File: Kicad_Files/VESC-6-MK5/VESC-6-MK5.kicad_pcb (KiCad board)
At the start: 4 copper layers, 105.9 x 102.5 mm, 151 parts, among them P1 USB_OTG, P10 PH_C, P11 SUPPLY, P12 GND, P2 CAN, P4 HALL_ENC, P5 COMM, P6 SERVO, P7 SWD, P8 PH_A, P9 PH_B, Q1 IRF7749, Q2 IRF7749, Q3 IRF7749, Q4 IRF7749, Q5 IRF7749, Q6 IRF7749, Q7 DMN62D0UW-7, U1 STM32F405RGTx, U10 MC74VHC1GT66, U11 SENS_VOLT, U12 MC74VHC1GT66, U13 MC74VHC1GT66, U14 MC74VHC1GT66DF1G, U15 MC74VHC1GT66DF1G, U16 MC74VHC1GT66DF1G, U3 DRV8301DCA, U4 TJA1051TK-3, U5 AD8418, U6 AD8418, U7 AD8418, U8 TC2117-3.3VEBTR, U9 BMI160, Y1 8M

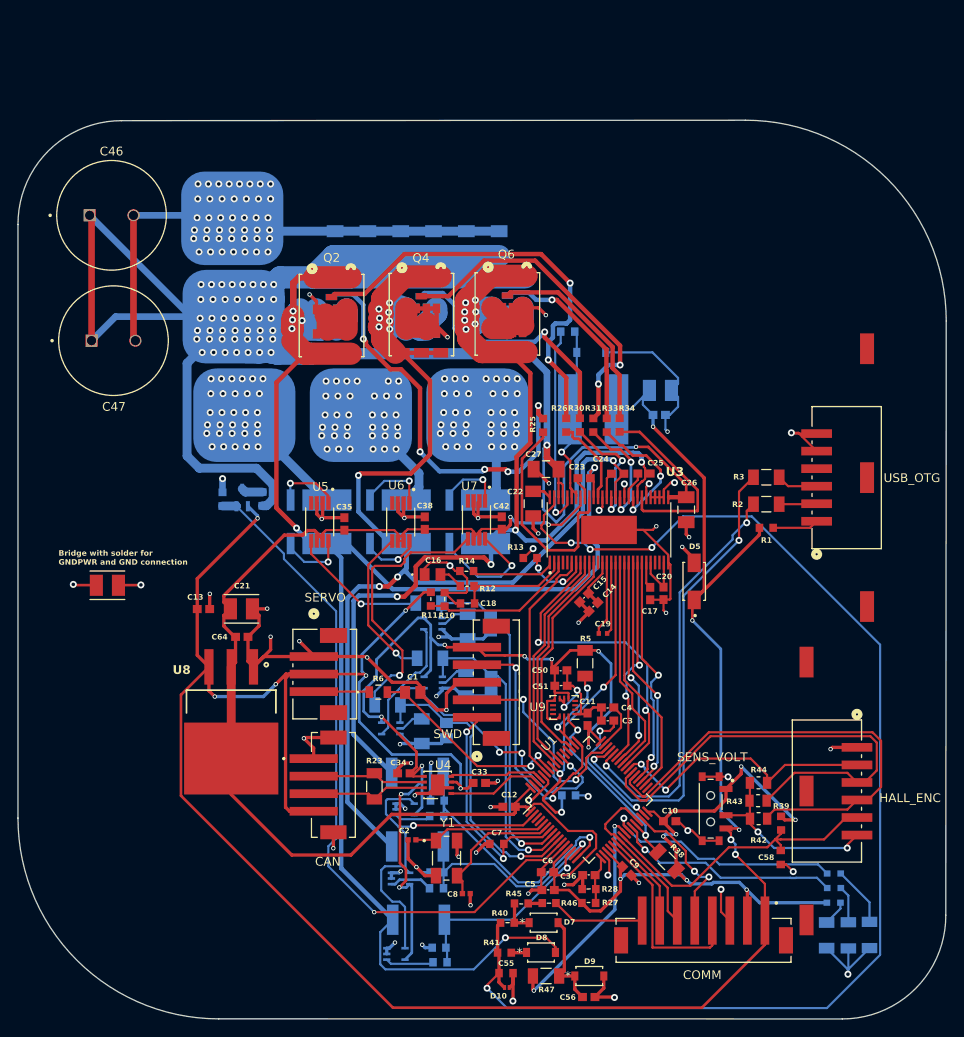
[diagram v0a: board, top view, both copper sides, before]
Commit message: Switched stunt resistors location
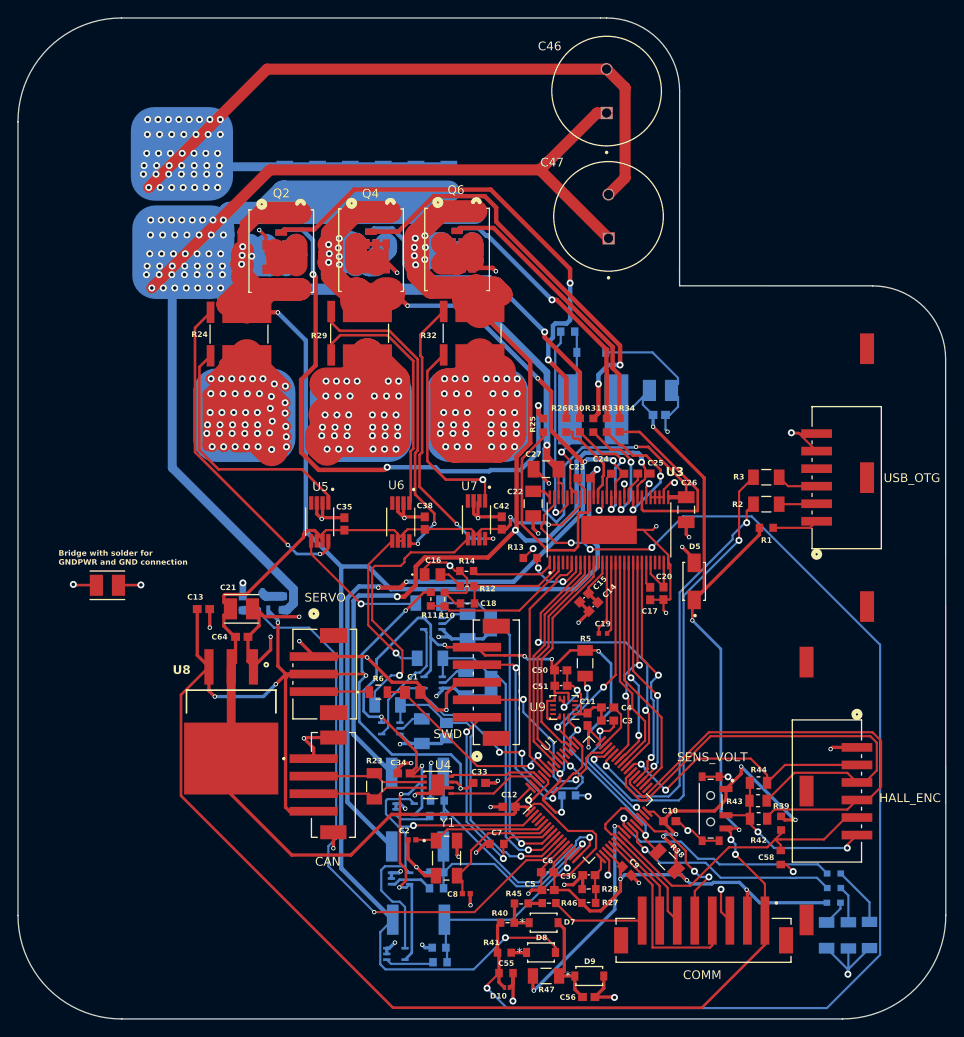
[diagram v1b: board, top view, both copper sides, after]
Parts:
- R24, R29, R32: moved to F.Cu
- moved C46 58.2 mm to (208.1, 46.6), turned to 90 degrees
- moved C47 58.2 mm to (208.3, 60.9), turned to 90 degrees
- moved R24 23.3 mm to (166.2, 74.3), turned to 90 degrees
- moved R29 21.9 mm to (179.9, 74.2), turned to 90 degrees
- moved R32 21.5 mm to (192.8, 74.2), turned to 90 degrees
- moved Q7 12.1 mm to (168.9, 104.9)
- moved R15 12.1 mm to (171.2, 105.0)
- moved R16 12.1 mm to (166.6, 105.0)
- moved Q5 9.34 mm to (191.1, 64.7)
- moved C37 9.33 mm to (171.4, 56.7)
- moved C39 9.33 mm to (175.1, 56.7)
- moved C40 9.33 mm to (178.9, 56.7)
- moved C41 9.33 mm to (182.6, 56.7)
- moved C43 9.33 mm to (186.4, 56.7)
- moved C44 9.33 mm to (190.1, 56.7)
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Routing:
- net Net-(P8-Pin_1): track 13.6 -> 210.7 mm, vias 31 -> 43
- net GNDPWR: track 135.5 -> 183.8 mm
- net SUPPLY: track 260.7 -> 306.9 mm
- net Net-(P9-Pin_1): track 13.0 -> 46.2 mm
- net /SH_A: track 184.6 -> 216.9 mm
- net Net-(U5-IN+): track 7.89 -> 37.8 mm, vias 1 -> 2
- net Net-(U6-IN+): track 6.92 -> 36.8 mm, vias 1 -> 2
- net Net-(P10-Pin_1): track 11.1 -> 40.4 mm
- net Net-(U5-IN-): track 7.65 -> 29.0 mm, vias 1 -> 0
- net Net-(U6-IN-): track 8.23 -> 28.6 mm, vias 1 -> 0
- net Net-(U7-IN+): track 13.9 -> 33.1 mm, vias 1 -> 2
- net Net-(Q1-G): track 47.0 -> 65.4 mm, vias 5 -> 3
- net Net-(U7-IN-): track 7.76 -> 22.6 mm
- net /DRV8301/SH_C: track 133.8 -> 146.5 mm, vias 11 -> 10
- net /DRV8301/SENS_SUPPLY: track 79.8 -> 69.3 mm
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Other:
- board size 105.9 x 102.5 mm -> 105.8 x 114.1 mm
